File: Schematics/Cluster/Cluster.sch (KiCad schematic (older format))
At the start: 49 parts, among them J1 FairingConnector, J10 PowerReg, J11 Conn_01x02, J12 Conn_01x03, J13 ClkOUT, J2 Serial, J3 i2c, J4 Programming, J5 GPIO, J6 Conn_01x07, J7 Conn_01x40, J8 Conn_01x40, J9 Conn_01x03, U1 LIS3DHTR, U2 LM2596S-ADJ, U3 STM32F411RETx, U4 AiP8563, U5 badge-rescue_HX4056, Y1 8MHz, Y2 32.768kHz

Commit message: Finished design for turnsignal/taillight assembly
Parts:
- added C17, C18, C19, C20, C21: 100nF, Capacitors_SMD:C_0805, symbol Device:C_Small
- added D4, D5, D6, D7, D8: SK6812, LEDs:LED_WS2812B-PLCC4, symbol LED:SK6812
- added R8: 1.5, Resistors_SMD:R_0805, symbol Device:R_Small
- BT1: footprint (none) -> Battery_Holders:Keystone_3008_1x2450-CoinCell
- C11, C12, C13, C14, C15, C16: footprint (none) -> Capacitors_SMD:C_0805
- D2, D3: footprint (none) -> Diodes_SMD:D_0603
- J13: footprint (none) -> Pin_Headers:Pin_Header_Straight_1x01_Pitch2.54mm
- J14: renamed from J?; footprint (none) -> TerminalBlock_RND:TerminalBlock_RND_205-00001_Pitch5.00mm
- R7: footprint (none) -> Resistors_SMD:R_0805
- U4: footprint (none) -> Housings_SSOP:MSOP-8_3x3mm_Pitch0.65mm; symbol Cluster:AiP8563 -> Cluster-rescue:AiP8563-Cluster
- U5: footprint (none) -> Badge:HX4056
- Y2: footprint (none) -> Crystals:Crystal_SMD_3215-2pin_3.2x1.5mm
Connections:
- net labels added: Neo
- wire segments 97 -> 130
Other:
- moved on the sheet: C10, C6, C7, C8, C9, R5, R6, U3, Y1

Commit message: Ordered V2
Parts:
- removed C10: 100nF, Capacitors_SMD:C_0805, symbol Device:C_Small
- removed J1: FairingConnector, TerminalBlock_RND:TerminalBlock_RND_205-00022_Pitch5.00mm, symbol Connector_Generic:Conn_01x12
- removed J4: Programming, Pin_Headers:Pin_Header_Straight_1x07_Pitch2.54mm, symbol Connector_Generic:Conn_01x07
- removed J6: Conn_01x07, Pin_Headers:Pin_Header_Straight_1x07_Pitch2.54mm, symbol Connector_Generic:Conn_01x07
- removed R5, R6: 100k, Resistors_SMD:R_0805, symbol Device:R_Small
- added C11, C14, C4, C5, C7, C9: 100nF, Capacitor_SMD:C_0805_2012Metric, symbol Device:C_Small
- added C17: 4.7uF, Capacitor_SMD:C_0805_2012Metric, symbol Device:C_Small
- added C23, C24: 1.5pF, Capacitor_SMD:C_0805_2012Metric, symbol Device:C_Small
- added C8: 1uF, Capacitor_SMD:C_0805_2012Metric, symbol Device:C_Small
- added D4: Pwr Ind, LED_SMD:LED_0603_1608Metric, symbol Device:LED_Small
- added J1: FairingConnector, TerminalBlock_RND:TerminalBlock_RND_205-00021_1x11_P5.00mm_Horizontal, symbol Connector_Generic:Conn_01x11
- added J15: Conn_01x02, TerminalBlock_RND:TerminalBlock_RND_205-00012_1x02_P5.00mm_Horizontal, symbol Connector_Generic:Conn_01x02
- added J4: Programming, Connector_PinHeader_2.54mm:PinHeader_1x08_P2.54mm_Vertical, symbol Connector_Generic:Conn_01x08
- added J6: Conn_01x06, Connector_PinHeader_2.54mm:PinHeader_1x06_P2.54mm_Vertical, symbol Connector_Generic:Conn_01x06
- added L2: L_Small, Inductor_SMD:L_0603_1608Metric, symbol Device:L_Small
- added R7: 330, Resistor_SMD:R_0603_1608Metric, symbol Device:R_Small
- added Y3: 32.768kHz, Crystal:Crystal_SMD_2012-2Pin_2.0x1.2mm, symbol Cluster-rescue:Crystal_Small-Device
- BT1: symbol Device:Battery_Cell -> Cluster-rescue:Battery_Cell-Device
- C1: footprint Capacitors_SMD:CP_Elec_8x10.5 -> Capacitor_SMD:CP_Elec_8x10.5; symbol Device:CP1 -> Cluster-rescue:CP1-Device
- C10: renamed from C2; footprint Capacitors_SMD:C_0805 -> Capacitor_SMD:C_0805_2012Metric; symbol Device:C_Small -> Cluster-rescue:C_Small-Device
- C12: renamed from C3; footprint Capacitors_SMD:C_0805 -> Capacitor_SMD:C_0805_2012Metric; symbol Device:C_Small -> Cluster-rescue:C_Small-Device
- C13: renamed from C14; footprint Capacitors_SMD:C_0805 -> Capacitor_SMD:C_0805_2012Metric; symbol Device:C_Small -> Cluster-rescue:C_Small-Device
- C15, C16: footprint Capacitors_SMD:C_0805 -> Capacitor_SMD:C_0805_2012Metric; symbol Device:C_Small -> Cluster-rescue:C_Small-Device
- C18: renamed from C4; footprint Capacitors_SMD:CP_Elec_8x10.5 -> Capacitor_SMD:CP_Elec_8x10.5; symbol Device:CP1 -> Cluster-rescue:CP1-Device
- C19: renamed from C5; footprint Capacitors_SMD:C_0805 -> Capacitor_SMD:C_0805_2012Metric; symbol Device:C_Small -> Cluster-rescue:C_Small-Device
- C2: renamed from C11; footprint Capacitors_SMD:C_0805 -> Capacitor_SMD:C_0805_2012Metric; symbol Device:C_Small -> Cluster-rescue:C_Small-Device
- C20: renamed from C17; footprint Capacitors_SMD:C_0805 -> Capacitor_SMD:C_0805_2012Metric; symbol Device:C_Small -> Cluster-rescue:C_Small-Device
- C21: renamed from C6; footprint Capacitors_SMD:C_0805 -> Capacitor_SMD:C_0805_2012Metric; symbol Device:C_Small -> Cluster-rescue:C_Small-Device
- C22: renamed from C7; footprint Capacitors_SMD:C_0805 -> Capacitor_SMD:C_0805_2012Metric; symbol Device:C_Small -> Cluster-rescue:C_Small-Device
- C25: renamed from C8; footprint Capacitors_SMD:C_0805 -> Capacitor_SMD:C_0805_2012Metric; symbol Device:C_Small -> Cluster-rescue:C_Small-Device
- C26: renamed from C9; footprint Capacitors_SMD:C_0805 -> Capacitor_SMD:C_0805_2012Metric; symbol Device:C_Small -> Cluster-rescue:C_Small-Device
- C27: renamed from C18; footprint Capacitors_SMD:C_0805 -> Capacitor_SMD:C_0805_2012Metric; symbol Device:C_Small -> Cluster-rescue:C_Small-Device
- C28: renamed from C19; footprint Capacitors_SMD:C_0805 -> Capacitor_SMD:C_0805_2012Metric; symbol Device:C_Small -> Cluster-rescue:C_Small-Device
- C29: renamed from C20; footprint Capacitors_SMD:C_0805 -> Capacitor_SMD:C_0805_2012Metric; symbol Device:C_Small -> Cluster-rescue:C_Small-Device
- C3: renamed from C12; footprint Capacitors_SMD:C_0805 -> Capacitor_SMD:C_0805_2012Metric; symbol Device:C_Small -> Cluster-rescue:C_Small-Device
- C30: renamed from C21; footprint Capacitors_SMD:C_0805 -> Capacitor_SMD:C_0805_2012Metric; symbol Device:C_Small -> Cluster-rescue:C_Small-Device
- C6: renamed from C13; footprint Capacitors_SMD:C_0805 -> Capacitor_SMD:C_0805_2012Metric; symbol Device:C_Small -> Cluster-rescue:C_Small-Device
- D1: symbol Diode:1N5822 -> Cluster-rescue:1N5822-Diode
- D2, D3: symbol Device:D_ALT -> Cluster-rescue:D_ALT-Device
- D5: renamed from D4; symbol LED:SK6812 -> Cluster-rescue:SK6812-LED
- D6: renamed from D5; symbol LED:SK6812 -> Cluster-rescue:SK6812-LED
- D7: renamed from D6; symbol LED:SK6812 -> Cluster-rescue:SK6812-LED
- D8: renamed from D7; symbol LED:SK6812 -> Cluster-rescue:SK6812-LED
- D9: renamed from D8; symbol LED:SK6812 -> Cluster-rescue:SK6812-LED
- J10: renamed from J9; footprint Pin_Headers:Pin_Header_Straight_1x03_Pitch2.54mm -> Connector_PinHeader_2.54mm:PinHeader_1x03_P2.54mm_Vertical; symbol Connector_Generic:Conn_01x03 -> Cluster-rescue:Conn_01x03-Connector_Generic
- J11: footprint Pin_Headers:Pin_Header_Straight_1x02_Pitch2.54mm -> Connector_PinHeader_2.54mm:PinHeader_1x02_P2.54mm_Vertical; symbol Connector_Generic:Conn_01x02 -> Cluster-rescue:Conn_01x02-Connector_Generic
- J12: renamed from J10; footprint Pin_Headers:Pin_Header_Straight_1x01_Pitch2.54mm -> Connector_PinHeader_2.54mm:PinHeader_1x01_P2.54mm_Vertical; symbol Connector_Generic:Conn_01x01 -> Cluster-rescue:Conn_01x01-Connector_Generic
- J13: renamed from J12; footprint Pin_Headers:Pin_Header_Straight_1x03_Pitch2.54mm -> Connector_PinHeader_2.54mm:PinHeader_1x03_P2.54mm_Vertical; symbol Connector_Generic:Conn_01x03 -> Cluster-rescue:Conn_01x03-Connector_Generic
- J14: renamed from J13; footprint Pin_Headers:Pin_Header_Straight_1x01_Pitch2.54mm -> Connector_PinHeader_2.54mm:PinHeader_1x01_P2.54mm_Vertical; symbol Connector_Generic:Conn_01x01 -> Cluster-rescue:Conn_01x01-Connector_Generic
- J2, J3: footprint Pin_Headers:Pin_Header_Straight_1x03_Pitch2.54mm -> Connector_PinHeader_2.54mm:PinHeader_1x03_P2.54mm_Vertical; symbol Connector_Generic:Conn_01x03 -> Cluster-rescue:Conn_01x03-Connector_Generic
- J5: footprint Pin_Headers:Pin_Header_Straight_1x06_Pitch2.54mm -> Connector_PinHeader_2.54mm:PinHeader_1x06_P2.54mm_Vertical; symbol Connector_Generic:Conn_01x06 -> Cluster-rescue:Conn_01x06-Connector_Generic
- J7: renamed from J8; footprint Connectors:XF2M -> Cluster:XF2M-4015; symbol Connector_Generic:Conn_01x40 -> Cluster-rescue:Conn_01x40-Connector_Generic
- J8: renamed from J14; symbol Connector_Generic:Conn_01x02 -> Cluster-rescue:Conn_01x02-Connector_Generic
- J9: renamed from J7; footprint Pin_Headers:Pin_Header_Straight_1x40_Pitch1.00mm -> Connector_PinHeader_1.00mm:PinHeader_1x40_P1.00mm_Vertical; symbol Connector_Generic:Conn_01x40 -> Cluster-rescue:Conn_01x40-Connector_Generic
- L1: symbol Device:L_Small -> Cluster-rescue:L_Small-Device
- R1: renamed from R8; symbol Device:R_Small -> Cluster-rescue:R_Small-Device
- R2: renamed from R3; symbol Device:R_Small -> Cluster-rescue:R_Small-Device
- R3: renamed from R7; symbol Device:R_Small -> Cluster-rescue:R_Small-Device
- R4: renamed from R1; symbol Device:R_Small -> Cluster-rescue:R_Small-Device
- R5: renamed from R2; symbol Device:R_Small -> Cluster-rescue:R_Small-Device
- R6: renamed from R4; symbol Device:R_Small -> Cluster-rescue:R_Small-Device
- U2: symbol Regulator_Switching:LM2596S-ADJ -> Cluster-rescue:LM2596S-ADJ-Regulator_Switching
- U4: renamed from U5; symbol badge-cache:badge-rescue_HX4056 -> Cluster-rescue:badge-rescue_HX4056-badge-cache
- U5: renamed from U3; symbol MCU_ST_STM32F4:STM32F411RETx -> Cluster-rescue:STM32F411RETx-MCU_ST_STM32F4
- Y1: renamed from Y2; symbol Device:Crystal_Small -> Cluster-rescue:Crystal_Small-Device
- Y2: renamed from Y1; symbol Device:Crystal -> Cluster-rescue:Crystal-Device
- renumbered U4 to U3
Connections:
- net +12V: now also J15.1 (Pin_1)
- net Fuel: now also J1.10 (Pin_10)
- net HighBeam: now also J1.3 (Pin_3)
- net JRST: now also J4.3 (Pin_3)
- net LeftTurn: now also J1.5 (Pin_5)
- net LightsOutAux: now also J6.4 (Pin_4)
- net LightsOutAuxTwo: now also J6.3 (Pin_3)
- net LightsOutBack: now also J6.5 (Pin_5)
- net LightsOutFront: now also J6.6 (Pin_6)
- net LowFuel: now also J1.7 (Pin_7)
- net Neutral: now also J1.11 (Pin_11)
- net Oil: now also J1.9 (Pin_9)
- net OverDrive: now also J1.6 (Pin_6)
- net Reset: now also J4.7 (Pin_7)
- net RightTurn: now also J1.4 (Pin_4)
- net SWCLK: now also J4.5 (Pin_5)
- net SWDIO: now also J4.6 (Pin_6)
- net SWO: now also J4.4 (Pin_4)
- net Temp: now also J1.8 (Pin_8)
- net VCC: now also J10.1 (Pin_1), J10.3 (Pin_3), J7.11 (Pin_11), J7.12 (Pin_12), J7.15 (Pin_15), J7.38 (Pin_38), J7.40 (Pin_40), J9.38 (Pin_38), J9.40 (Pin_40), C11.1, C14.1, C17.1, C4.1, C7.1, C9.1, J1.1 (Pin_1), J4.1 (Pin_1), J6.1 (Pin_1), L2.2, R7.1
- net VSS: now also J10.2 (Pin_2), J7.17 (Pin_17), J7.18 (Pin_18), J7.19 (Pin_19), J7.20 (Pin_20), J7.21 (Pin_21), J7.22 (Pin_22), J7.23 (Pin_23), J7.24 (Pin_24), J7.25 (Pin_25), J7.26 (Pin_26), J7.27 (Pin_27), J7.28 (Pin_28), J7.29 (Pin_29), J7.30 (Pin_30), J7.31 (Pin_31), J7.32 (Pin_32), J7.34 (Pin_34), J7.35 (Pin_35), J7.37 (Pin_37), J7.39 (Pin_39), J9.39 (Pin_39), C11.2, C14.2, C17.2, C23.2, C24.2, C4.2, C5.2, C7.2, C8.2, C9.2, D4.1 (K), J1.2 (Pin_2), J15.2 (Pin_2), J4.2 (Pin_2), J6.2 (Pin_2); no longer J7.9 (Pin_9)
- net VDDA: now reaches U5.13 (VDDA)
- net VDDA: now also C5.1, C8.1, L2.1
- net at U5.3 (PC14): now also C23.1, Y3.1
- net at U5.4 (PC15): now also C24.1, Y3.2
- net Boot0: now reaches U5.60 (BOOT0)
- net Boot0: now also J4.8 (Pin_8)
- net at J9.1 (Pin_1): no longer J7.1 (Pin_1)
- net at J9.11 (Pin_11): no longer J7.11 (Pin_11)
- net at J9.12 (Pin_12): no longer J7.12 (Pin_12)
- net at J9.15 (Pin_15): no longer J7.15 (Pin_15)
- net at J9.17 (Pin_17): no longer J7.17 (Pin_17)
- net at J9.18 (Pin_18): no longer J7.18 (Pin_18)
- net at J9.19 (Pin_19): no longer J7.19 (Pin_19)
- net at J9.2 (Pin_2): no longer J7.2 (Pin_2)
- net at J9.20 (Pin_20): no longer J7.20 (Pin_20)
- net at J9.21 (Pin_21): no longer J7.21 (Pin_21)
- net at J9.22 (Pin_22): no longer J7.22 (Pin_22)
- net at J9.23 (Pin_23): no longer J7.23 (Pin_23)
- net at J9.24 (Pin_24): no longer J7.24 (Pin_24)
- net at J9.25 (Pin_25): no longer J7.25 (Pin_25)
- net at J9.26 (Pin_26): no longer J7.26 (Pin_26)
- net at J9.27 (Pin_27): no longer J7.27 (Pin_27)
- net at J9.28 (Pin_28): no longer J7.28 (Pin_28)
- net at J9.29 (Pin_29): no longer J7.29 (Pin_29)
- net at J9.3 (Pin_3): no longer J7.3 (Pin_3)
- net at J9.30 (Pin_30): no longer J7.30 (Pin_30)
- net at J9.31 (Pin_31): no longer J7.31 (Pin_31)
- net at J9.32 (Pin_32): no longer J7.32 (Pin_32)
- net at J9.34 (Pin_34): no longer J7.34 (Pin_34)
- net at J9.35 (Pin_35): no longer J7.35 (Pin_35)
- net at J9.37 (Pin_37): no longer J7.37 (Pin_37)
- net at J9.4 (Pin_4): no longer J7.4 (Pin_4)
- net at J9.8 (Pin_8): no longer J7.8 (Pin_8)
- new net: D4.2 (A), R7.2
- no-connect marks 20 -> 51
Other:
- moved on the sheet: D3, J10, J7, J9

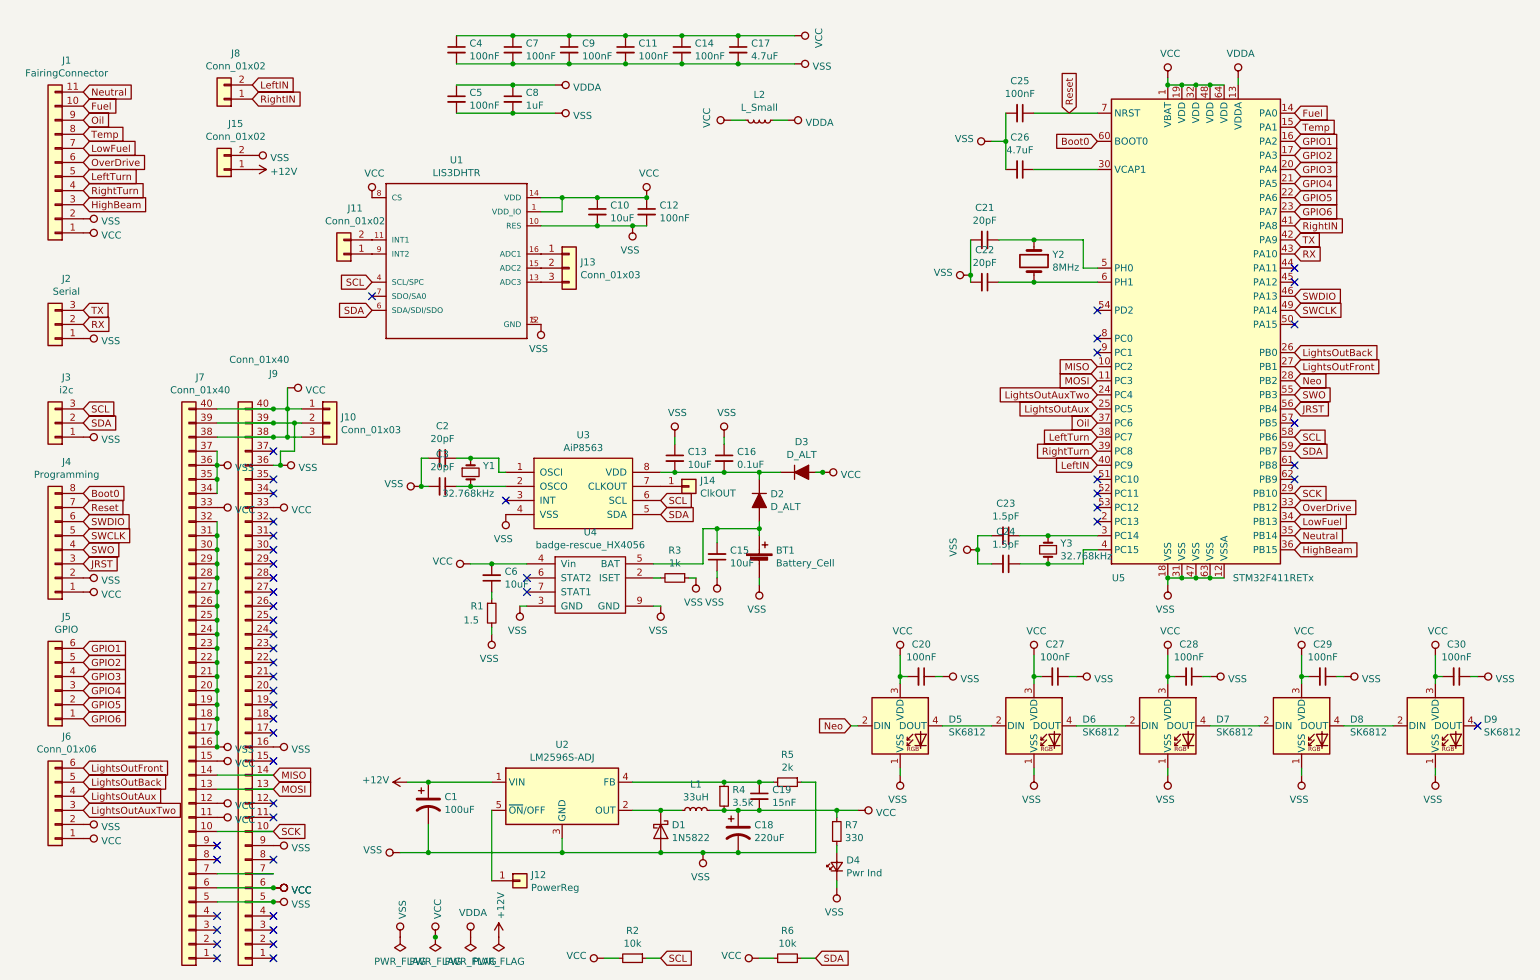
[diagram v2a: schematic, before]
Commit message: Why are there still ratsnest wires?
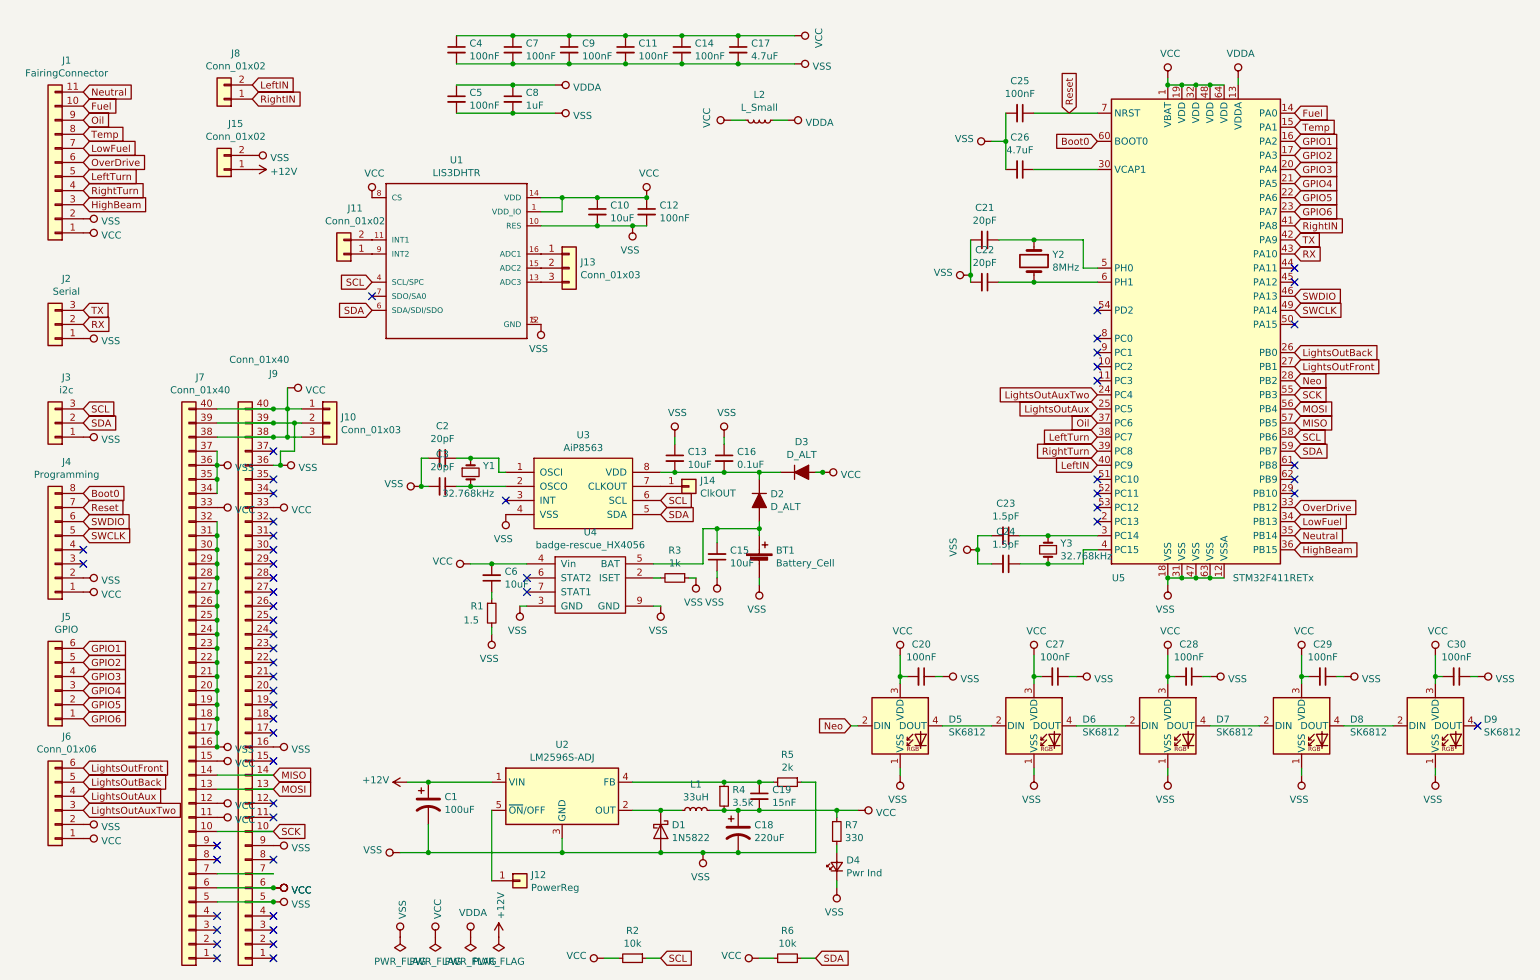
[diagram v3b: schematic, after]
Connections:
- net MISO: now also U5.57 (PB5); no longer U5.10 (PC2)
- net MOSI: now also U5.56 (PB4); no longer U5.11 (PC3)
- net SCK: now also U5.55 (PB3); no longer U5.29 (PB10)
- net JRST: no longer names the net of J4.3 (Pin_3)
- net JRST: no longer U5.56 (PB4)
- net SWO: no longer names the net of J4.4 (Pin_4)
- net SWO: no longer U5.55 (PB3)
- no-connect marks 51 -> 55
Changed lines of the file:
@@
 Text GLabel 9650 2950 2    50   Input ~ 0
 SWCLK
-Text GLabel 9650 3550 2    50   Input ~ 0
-SWO
-Text GLabel 9650 3650 2    50   Input ~ 0
-JRST
-Text GLabel 1050 4650 2    50   Input ~ 0
-SWO
-Text GLabel 1050 4750 2    50   Input ~ 0
-JRST
 Text GLabel 1050 4450 2    50   Input ~ 0
 SWDIO
@@
 	0    1    1    0
 $EndComp
-Text GLabel 8250 3350 0    50   Input ~ 0
-MISO
-Text GLabel 8250 3450 0    50   Input ~ 0
-MOSI
-Text GLabel 9650 4250 2    50   Input ~ 0
-SCK
 Text GLabel 2400 6650 2    50   Input ~ 0
 SCK
@@
 NoConn ~ 9650 4150
 NoConn ~ 9650 4050
-NoConn ~ 9650 3750
 NoConn ~ 9650 3050
 NoConn ~ 9650 2650
@@
 	1    0    0    -1
 $EndComp
-Connection ~ 3550 7400
 $Comp
 L Cluster-rescue:+12V-power #PWR032
@@
 	-1   0    0    1
 $EndComp
+Text GLabel 9650 3550 2    50   Input ~ 0
+SCK
+Text GLabel 9650 3750 2    50   Input ~ 0
+MISO
+Text GLabel 9650 3650 2    50   Input ~ 0
+MOSI
+NoConn ~ 9650 4250
+NoConn ~ 8250 3450
+NoConn ~ 8250 3350
+NoConn ~ 1050 4650
+NoConn ~ 1050 4750
 $EndSCHEMATC
